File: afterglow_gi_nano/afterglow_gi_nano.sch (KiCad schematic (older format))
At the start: 16 parts

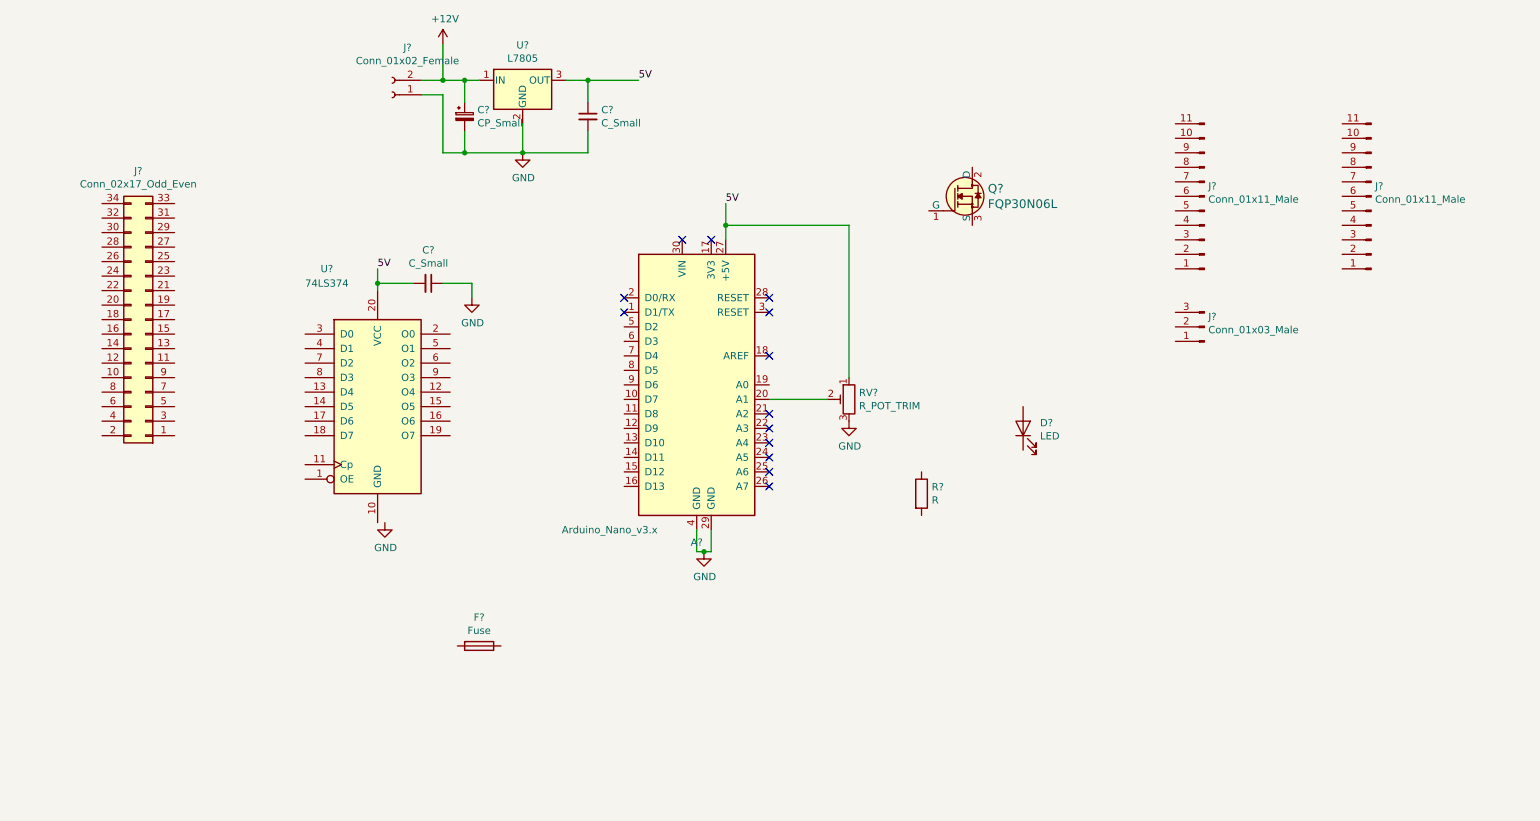
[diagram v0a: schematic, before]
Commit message: Schematic progress
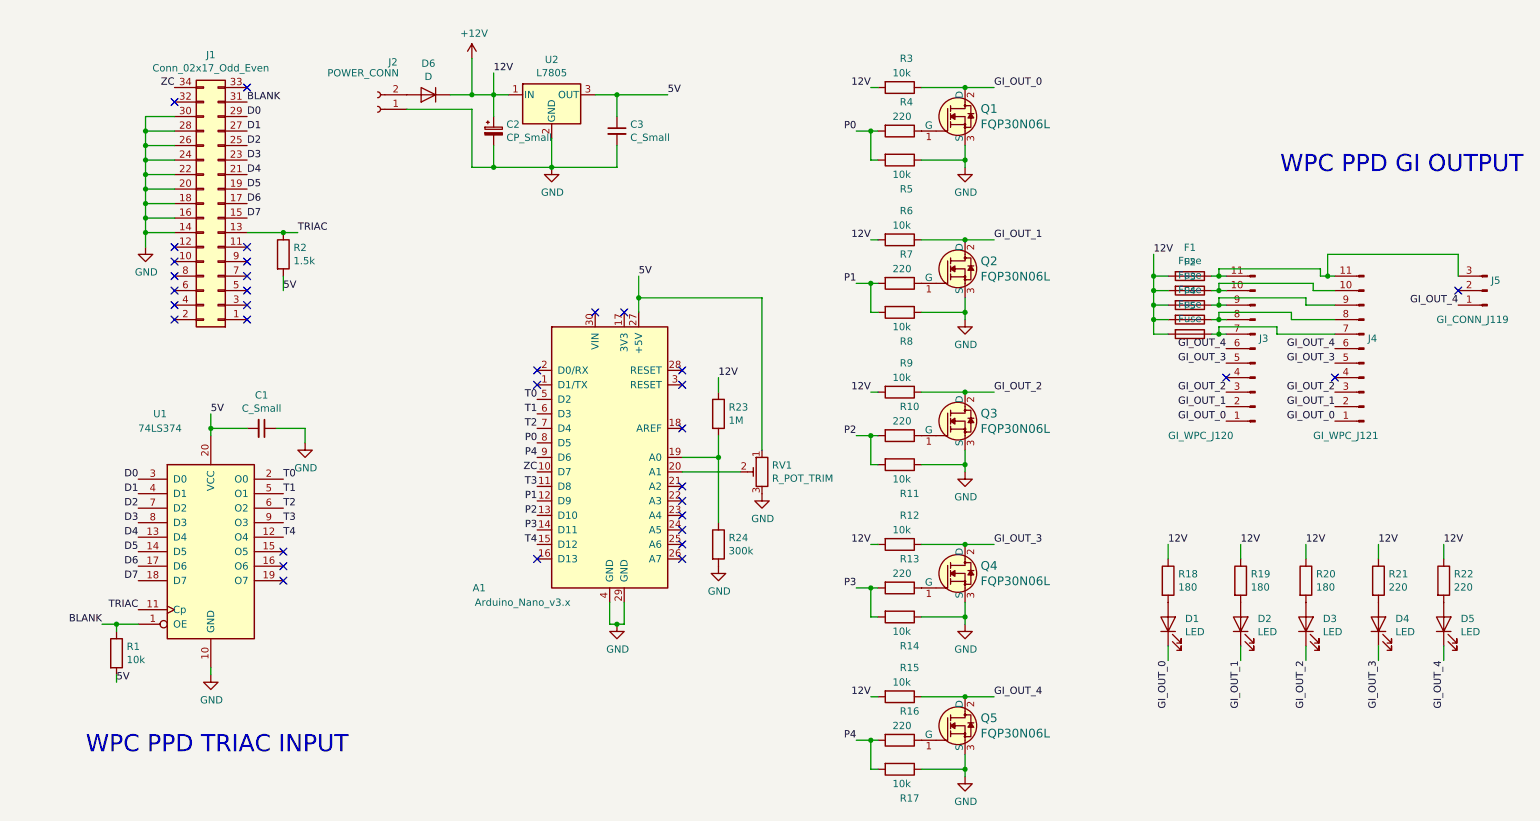
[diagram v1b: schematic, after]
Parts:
- added D2, D3, D4, D5: LED, symbol Device:LED
- added D6: D, symbol Device:D
- added F2, F3, F4, F5: Fuse, symbol Device:Fuse
- added Q2, Q3, Q4, Q5: FQP30N06L, digikey-footprints:TO-220-3, symbol dk_Transistors-FETs-MOSFETs-Single:FQP30N06L
- added R10, R13, R16, R21, R22, R4, R7: 220, symbol Device:R
- added R11, R12, R14, R15, R17, R3, R5, R6, R8, R9: 10k, symbol Device:R
- added R18, R19, R20: 180, symbol Device:R
- added R2: 1.5k, symbol Device:R
- added R23: 1M, symbol Device:R
- added R24: 300k, symbol Device:R
- J2: renamed from J?; value Conn_01x02_Female -> POWER_CONN
- J3: renamed from J?; value Conn_01x11_Male -> GI_WPC_J120
- J4: renamed from J?; value Conn_01x11_Male -> GI_WPC_J121
- J5: renamed from J?; value Conn_01x03_Male -> GI_CONN_J119
- R1: renamed from R?; value R -> 10k
- gave numbers to parts that had none: 11
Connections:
- net +12V: now also F1.2, D6.1 (K), F2.2, F3.2, F4.2, F5.2, R12.2, R15.2, R18.1, R19.1, R20.1, R21.1, R22.1, R23.1, R3.2, R6.2, R9.2; no longer J2.2 (Pin_2)
- net 5V: now also R1.2, R2.2
- net GND: now also J1.14 (Pin_14), J1.16 (Pin_16), J1.18 (Pin_18), J1.20 (Pin_20), J1.22 (Pin_22), J1.24 (Pin_24), J1.26 (Pin_26), J1.28 (Pin_28), J1.30 (Pin_30), Q1.3 (S), U1.10 (GND), Q2.3 (S), Q3.3 (S), Q4.3 (S), Q5.3 (S), R11.1, R14.1, R17.1, R24.2, R5.1, R8.1
- net ZC: now reaches A1.10 (D7)
- net ZC: now also J1.34 (Pin_34)
- net T3: now reaches A1.11 (D8)
- net T3: now also U1.9 (O3)
- net P1: now reaches A1.12 (D9)
- net P1: now also R7.2, R8.2
- net P2: now reaches A1.13 (D10)
- net P2: now also R10.2, R11.2
- net P3: now reaches A1.14 (D11)
- net P3: now also R13.2, R14.2
- net T4: now reaches A1.15 (D12)
- net T4: now also U1.12 (O4)
- net at A1.19 (A0): now also R23.2, R24.1
- net T0: now reaches A1.5 (D2)
- net T0: now also U1.2 (O0)
- net T1: now reaches A1.6 (D3)
- net T1: now also U1.5 (O1)
- net T2: now reaches A1.7 (D4)
- net T2: now also U1.6 (O2)
- net P0: now reaches A1.8 (D5)
- net P0: now also R4.2, R5.2
- net P4: now reaches A1.9 (D6)
- net P4: now also R16.2, R17.2
- net BLANK: now reaches U1.1 (OE)
- net BLANK: now also J1.31 (Pin_31), R1.1
- net TRIAC: now reaches U1.11 (Cp)
- net TRIAC: now also J1.13 (Pin_13), R2.1
- net D4: now reaches U1.13 (D4)
- net D4: now also J1.21 (Pin_21)
- net D5: now reaches U1.14 (D5)
- net D5: now also J1.19 (Pin_19)
- net D6: now reaches U1.17 (D6)
- net D6: now also J1.17 (Pin_17)
- net D7: now reaches U1.18 (D7)
- net D7: now also J1.15 (Pin_15)
- net D0: now reaches U1.3 (D0)
- net D0: now also J1.29 (Pin_29)
- net D1: now reaches U1.4 (D1)
- net D1: now also J1.27 (Pin_27)
- net D2: now reaches U1.7 (D2)
- net D2: now also J1.25 (Pin_25)
- net D3: now reaches U1.8 (D3)
- net D3: now also J1.23 (Pin_23)
- net at Q1.1 (G): now also R4.1
- net GI_OUT_0: now reaches Q1.2 (D)
- net GI_OUT_0: now also D1.1 (K), J3.1 (Pin_1), J4.1 (Pin_1), R3.1
- net at J3.10 (Pin_10): now also J4.10 (Pin_10), F2.1
- net at J3.11 (Pin_11): now also F1.1, J4.11 (Pin_11), J5.3 (Pin_3)
- net GI_OUT_1: now reaches J3.2 (Pin_2)
- net GI_OUT_1: now also J4.2 (Pin_2), D2.1 (K), Q2.2 (D), R6.1
- net GI_OUT_2: now reaches J3.3 (Pin_3)
- net GI_OUT_2: now also J4.3 (Pin_3), D3.1 (K), Q3.2 (D), R9.1
- net GI_OUT_3: now reaches J3.5 (Pin_5)
- net GI_OUT_3: now also J4.5 (Pin_5), D4.1 (K), Q4.2 (D), R12.1
- net GI_OUT_4: now reaches J3.6 (Pin_6)
- net GI_OUT_4: now also J4.6 (Pin_6), J5.1 (Pin_1), D5.1 (K), Q5.2 (D), R15.1
- net at J3.7 (Pin_7): now also J4.7 (Pin_7), F5.1
- net at J3.8 (Pin_8): now also J4.8 (Pin_8), F4.1
- net at J3.9 (Pin_9): now also J4.9 (Pin_9), F3.1
- net at D1.2 (A): now also R18.2
- new net: D6.2 (A), J2.2 (Pin_2)
- new net: D2.2 (A), R19.2
- new net: D3.2 (A), R20.2
- new net: D4.2 (A), R21.2
- new net: D5.2 (A), R22.2
- new net: Q2.1 (G), R7.1
- new net: Q3.1 (G), R10.1
- new net: Q4.1 (G), R13.1
- new net: Q5.1 (G), R16.1
- no-connect marks 13 -> 34
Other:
- note added: "WPC PPD GI OUTPUT"
- note added: "WPC PPD TRIAC INPUT"
- moved on the sheet: A1, C1, C2, C3, D1, F1, J1, J2, J3, J4, J5, Q1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

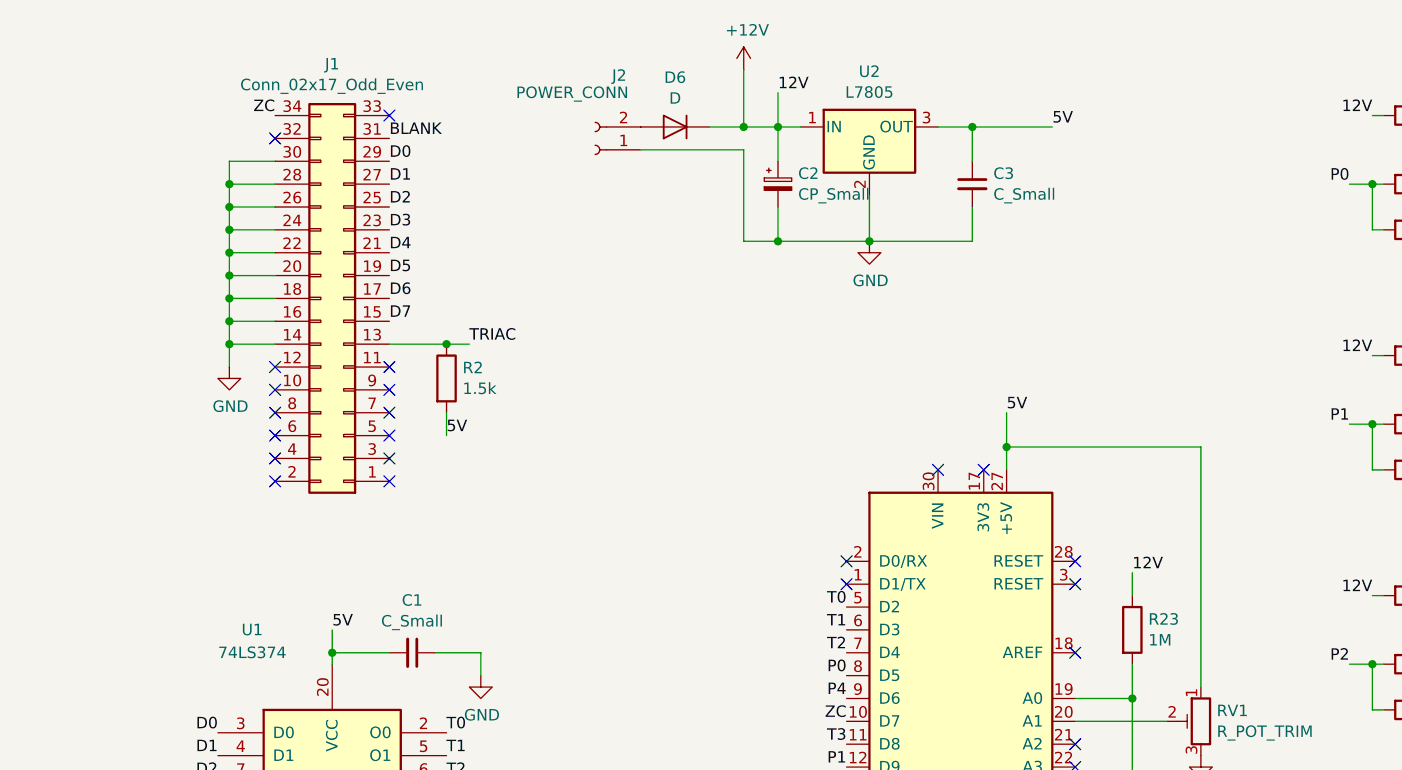
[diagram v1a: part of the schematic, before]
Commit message: Schematic progressing
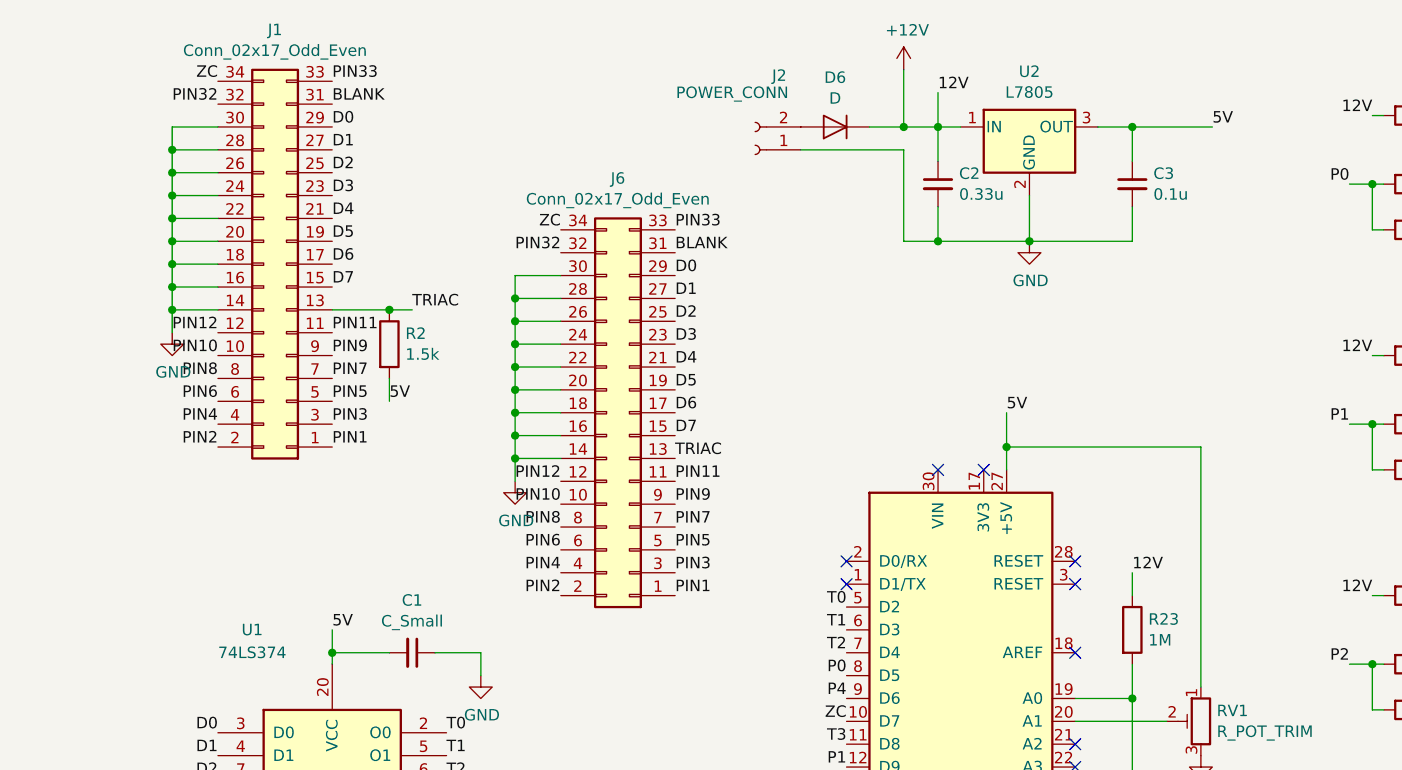
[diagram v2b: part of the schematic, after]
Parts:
- removed C2: CP_Small, symbol Device:CP_Small
- added C2: 0.33u, Capacitors_SMD:C_0805_HandSoldering, symbol Device:C_Small
- added J6: Conn_02x17_Odd_Even, Pin_Headers:Pin_Header_Straight_2x17_Pitch2.54mm, symbol Connector_Generic:Conn_02x17_Odd_Even
- C1: footprint (none) -> Capacitors_SMD:C_0805_HandSoldering
- C3: value C_Small -> 0.1u; footprint (none) -> Capacitors_SMD:C_0805_HandSoldering
- D1, D2, D3, D4, D5: footprint (none) -> LEDs:LED_0805_HandSoldering
- D6: footprint (none) -> Diodes_THT:D_5W_P10.16mm_Horizontal
- F1, F2, F3, F4, F5: footprint (none) -> Fuse_Holders_and_Fuses:Fuseholder5x20_horiz_open_lateral_Type-II
- J1: footprint (none) -> Connectors:IDC_Header_Straight_34pins
- J2: footprint (none) -> Connectors_Molex:Molex_KK-41791-02_02x3.96mm_Straight
- J3, J4: footprint (none) -> Connectors_Molex:Molex_KK-41791-11_10x3.96mm_Straight
- J5: footprint (none) -> Connectors_Molex:Molex_KK-41791-03_03x3.96mm_Straight
- Q1, Q2, Q3, Q4, Q5: footprint digikey-footprints:TO-220-3 -> TO_SOT_Packages_THT:TO-220_Vertical
- R1, R10, R11, R12, R13, R14, R15, R16, R17, R18, R19, R2, R20, R21, R22, R23, R24, R3, R4, R5, R6, R7, R8, R9: footprint (none) -> Resistors_SMD:R_0805_HandSoldering
- RV1: footprint (none) -> Potentiometers:Potentiometer_Trimmer_Piher_PT-6v_Horizontal
- U1: footprint (none) -> Housings_DIP:DIP-20_W7.62mm_LongPads
- U2: footprint (none) -> TO_SOT_Packages_THT:TO-220_Vertical
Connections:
- net +12V: now also C2.1
- net BLANK: now also J6.31 (Pin_31)
- net D0: now also J6.29 (Pin_29)
- net D1: now also J6.27 (Pin_27)
- net D2: now also J6.25 (Pin_25)
- net D3: now also J6.23 (Pin_23)
- net D4: now also J6.21 (Pin_21)
- net D5: now also J6.19 (Pin_19)
- net D6: now also J6.17 (Pin_17)
- net D7: now also J6.15 (Pin_15)
- net GND: now also C2.2, J6.14 (Pin_14), J6.16 (Pin_16), J6.18 (Pin_18), J6.20 (Pin_20), J6.22 (Pin_22), J6.24 (Pin_24), J6.26 (Pin_26), J6.28 (Pin_28), J6.30 (Pin_30)
- net TRIAC: now also J6.13 (Pin_13)
- net ZC: now also J6.34 (Pin_34)
- net PIN1: now reaches J1.1 (Pin_1)
- net PIN1: now also J6.1 (Pin_1)
- net PIN10: now reaches J1.10 (Pin_10)
- net PIN10: now also J6.10 (Pin_10)
- net PIN11: now reaches J1.11 (Pin_11)
- net PIN11: now also J6.11 (Pin_11)
- net PIN12: now reaches J1.12 (Pin_12)
- net PIN12: now also J6.12 (Pin_12)
- net PIN2: now reaches J1.2 (Pin_2)
- net PIN2: now also J6.2 (Pin_2)
- net PIN3: now reaches J1.3 (Pin_3)
- net PIN3: now also J6.3 (Pin_3)
- net PIN32: now reaches J1.32 (Pin_32)
- net PIN32: now also J6.32 (Pin_32)
- net PIN33: now reaches J1.33 (Pin_33)
- net PIN33: now also J6.33 (Pin_33)
- net PIN4: now reaches J1.4 (Pin_4)
- net PIN4: now also J6.4 (Pin_4)
- net PIN5: now reaches J1.5 (Pin_5)
- net PIN5: now also J6.5 (Pin_5)
- net PIN6: now reaches J1.6 (Pin_6)
- net PIN6: now also J6.6 (Pin_6)
- net PIN7: now reaches J1.7 (Pin_7)
- net PIN7: now also J6.7 (Pin_7)
- net PIN8: now reaches J1.8 (Pin_8)
- net PIN8: now also J6.8 (Pin_8)
- net PIN9: now reaches J1.9 (Pin_9)
- net PIN9: now also J6.9 (Pin_9)
- no-connect marks 34 -> 20
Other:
- moved on the sheet: C3, D6, J1, J2, R2, U2
